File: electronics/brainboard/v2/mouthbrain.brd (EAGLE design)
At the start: 101.6 x 53.3 mm, 28 parts, among them Q1 MOSFET-NCHANNELSMD, Q10 MOSFET-NCHANNELSMD, Q11 MOSFET-NCHANNELSMD, Q12 MOSFET-NCHANNELSMD, Q13 MOSFET-NCHANNELSMD, Q14 MOSFET-NCHANNELSMD, Q15 MOSFET-NCHANNELSMD, Q16 MOSFET-NCHANNELSMD, Q2 MOSFET-NCHANNELSMD, Q3 MOSFET-NCHANNELSMD, Q4 MOSFET-NCHANNELSMD, Q5 MOSFET-NCHANNELSMD, Q6 MOSFET-NCHANNELSMD, Q7 MOSFET-NCHANNELSMD, Q8 MOSFET-NCHANNELSMD, Q9 MOSFET-NCHANNELSMD, U2 ARDUINO-MEGAFULL

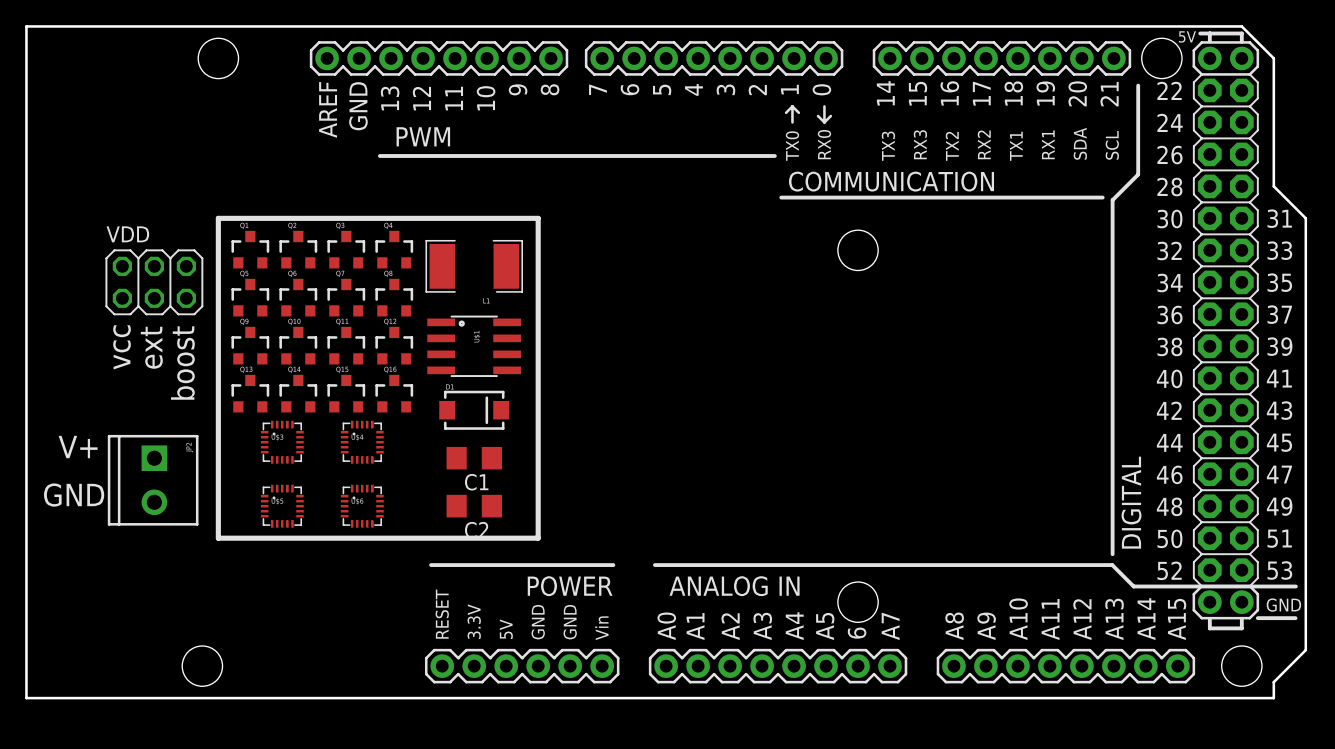
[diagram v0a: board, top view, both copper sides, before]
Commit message: circuit is ready to rock and roll.
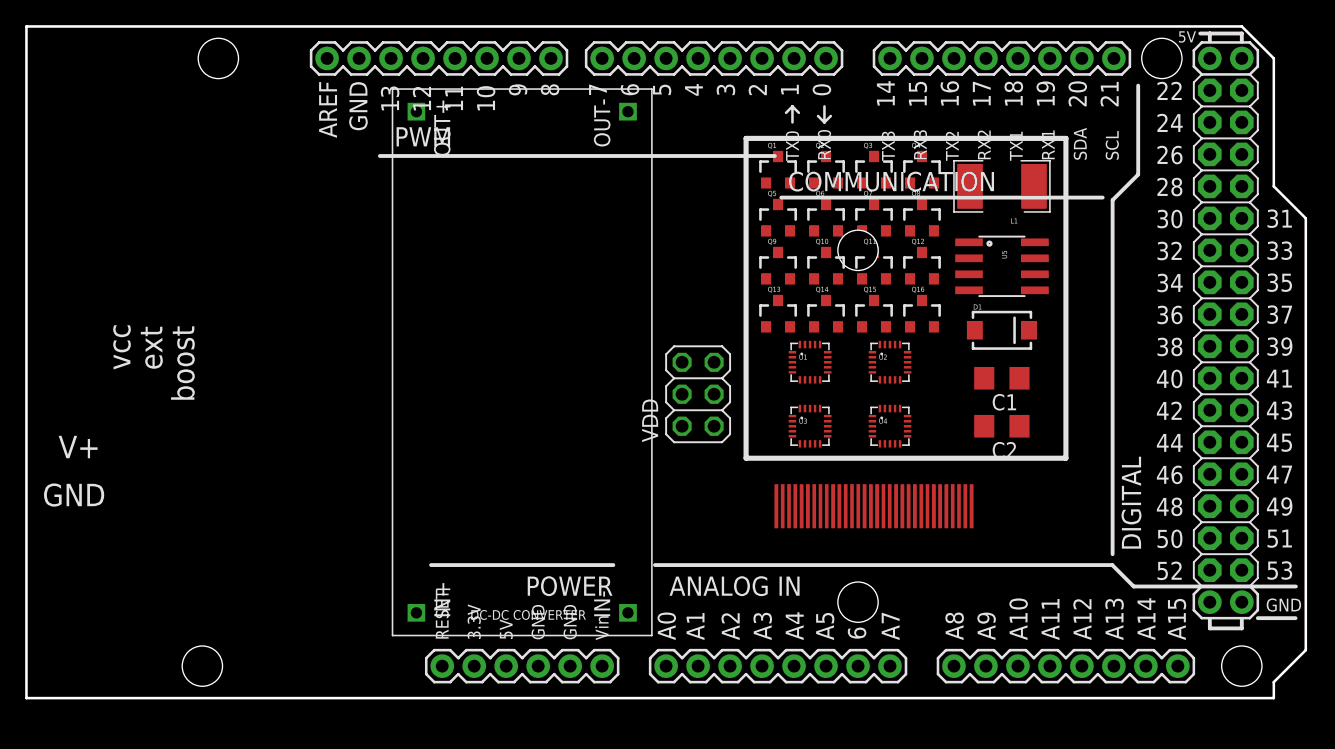
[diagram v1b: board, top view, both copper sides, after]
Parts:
- removed JP2: (no value), SparkFun:SCREWTERMINAL-3.5MM-2
- removed U$3, U$4, U$5, U$6: MCP4352, mouthbrain:QFN-20
- added MEGA: ARDUINO-MEGAFULL, SparkFun:ARDUINO_MEGA
- added U$2: FPC-0.5-32, Hoektronics:FPC-PCB-32
- added U1, U3, U4: MCP4352, mouthbrain:QFN-20
- added U5: MOSFET-NCHANNEL-SOIC8, SparkFun:SO08
- U$1: value MOSFET-NCHANNEL-SOIC8 -> DC-DC-CONVERTER; device SparkFun:SO08 -> Hoektronics:DC-DC-MODULE
- U2: value ARDUINO-MEGAFULL -> MCP4352; device SparkFun:ARDUINO_MEGA -> mouthbrain:QFN-20
- moved U2 73.6 mm to (68.6, 29.2)
- moved VDD 44.1 mm to (53.3, 26.7), turned to 90 degrees
- moved Q11 42.4 mm to (67.3, 36.8)
- moved Q12 42.4 mm to (71.1, 36.8)
- moved Q15 42.4 mm to (67.3, 33.0)
- moved Q16 42.4 mm to (71.1, 33.0)
- moved Q3 42.4 mm to (67.3, 44.5)
- moved Q4 42.4 mm to (71.1, 44.5)
- moved Q7 42.4 mm to (67.3, 40.6)
- moved Q8 42.4 mm to (71.1, 40.6)
- moved C1 42.4 mm to (77.5, 27.9)
- moved C2 42.4 mm to (77.5, 24.1)
- moved D1 42.4 mm to (77.5, 31.8)
- moved L1 42.4 mm to (77.5, 43.2)
- moved Q1 42.4 mm to (59.7, 44.5)
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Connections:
- removed net AN0: Q1.1, U2.22
- removed net AN1: Q2.1, U2.23
- removed net AN10: Q11.1, U2.32
- removed net AN11: Q12.1, U2.33
- removed net AN12: Q13.1, U2.34
- removed net AN13: Q14.1, U2.35
- removed net AN14: Q15.1, U2.36
- removed net AN15: Q16.1
- removed net AN2: Q3.1, U2.24
- removed net AN3: Q4.1, U2.25
- removed net AN4: Q5.1, U2.26
- removed net AN5: Q6.1, U2.27
- removed net AN6: Q7.1, U2.28
- removed net AN7: Q8.1, U2.29
- removed net AN8: Q9.1, U2.30
- removed net AN9: Q10.1, U2.31
- removed net ANODE0: Q1.3
- removed net ANODE1: Q2.3
- removed net ANODE10: Q11.3
- removed net ANODE11: Q12.3
- removed net ANODE12: Q13.3
- removed net ANODE13: Q14.3
- removed net ANODE14: Q15.3
- removed net ANODE15: Q16.3
- removed net ANODE2: Q3.3
- removed net ANODE3: Q4.3
- removed net ANODE4: Q5.3
- removed net ANODE5: Q6.3
- removed net ANODE6: Q7.3
- removed net ANODE7: Q8.3
- removed net ANODE8: Q9.3
- removed net ANODE9: Q10.3
- removed net N$3: C1.1, D1.C
- removed net OUT0: U$3.10, U2.A0
- removed net OUT1: U$3.7, U2.A1
- removed net OUT10: U$5.17, U2.A10
- removed net OUT11: U$5.20, U2.A11
- removed net OUT12: U$6.10, U2.A12
- removed net OUT13: U$6.7, U2.A13
- removed net OUT14: U$6.17, U2.A14
- removed net OUT15: U$6.20, U2.A15
- removed net OUT2: U$3.17, U2.A2
- removed net OUT3: U$3.20, U2.A3
- removed net OUT4: U$4.10, U2.A4
- removed net OUT5: U$4.7, U2.A5
- removed net OUT6: U$4.17, U2.A6
- removed net OUT7: U$4.20, U2.A7
- removed net OUT8: U$5.10, U2.A8
- removed net OUT9: U$5.7, U2.A9
- new net AOUT0: MEGA.A0, U$2.P$2, U1.10
- new net AOUT1: MEGA.A1, U$2.P$4, U1.7
- new net AOUT10: MEGA.A10, U$2.P$22, U3.17
- new net AOUT11: MEGA.A11, U$2.P$24, U3.20
- new net AOUT12: MEGA.A12, U$2.P$26, U4.10
- new net AOUT13: MEGA.A13, U$2.P$28, U4.7
- new net AOUT14: MEGA.A14, U$2.P$30, U4.17
- new net AOUT15: MEGA.A15, U$2.P$32, U4.20
- new net AOUT2: MEGA.A2, U$2.P$6, U1.17
- new net AOUT3: MEGA.A3, U$2.P$8, U1.20
- new net AOUT4: MEGA.A4, U$2.P$10, U2.10
- new net AOUT5: MEGA.A5, U$2.P$12, U2.7
- new net AOUT6: MEGA.A6, U$2.P$14, U2.17
- new net AOUT7: MEGA.A7, U$2.P$16, U2.20
- new net AOUT8: MEGA.A8, U$2.P$18, U3.10
- new net AOUT9: MEGA.A9, U3.7
- new net CIN0: MEGA.22, Q1.1
- new net CIN1: MEGA.23, Q2.1
- new net CIN10: MEGA.32, Q11.1
- new net CIN11: MEGA.33, Q12.1
- new net CIN12: MEGA.34, Q13.1
- new net CIN13: MEGA.35, Q14.1
- new net CIN14: MEGA.36, Q15.1
- new net CIN15: MEGA.37, Q16.1
- new net CIN2: MEGA.24, Q3.1
- new net CIN3: MEGA.25, Q4.1
- new net CIN4: MEGA.26, Q5.1
- new net CIN5: MEGA.27, Q6.1
- new net CIN6: MEGA.28, Q7.1
- new net CIN7: MEGA.29, Q8.1
- new net CIN8: MEGA.30, Q9.1
- new net CIN9: MEGA.31, Q10.1
- new net COUT0: Q1.3, U$2.P$1
- new net COUT1: Q2.3, U$2.P$3
- new net COUT10: Q11.3, U$2.P$21
- new net COUT11: Q12.3, U$2.P$23
- new net COUT12: Q13.3, U$2.P$25
- new net COUT13: Q14.3, U$2.P$27
- new net COUT14: Q15.3, U$2.P$29
- new net COUT15: Q16.3, U$2.P$31
- new net COUT2: Q3.3, U$2.P$5
- new net COUT3: Q4.3, U$2.P$7
- new net COUT4: Q5.3, U$2.P$9
- new net COUT5: Q6.3, U$2.P$11
- new net COUT6: Q7.3, U$2.P$13
- new net COUT7: Q8.3, U$2.P$15
- new net COUT8: Q9.3, U$2.P$17
- new net COUT9: Q10.3, U$2.P$19, U$2.P$20
- net !CS1: now also MEGA.6, U1.2; no longer U$3.2, U2.6
- net !CS2: now also MEGA.7, U2.2; no longer U$4.2, U2.7
- net !CS3: now also MEGA.8, U3.2; no longer U$5.2, U2.8
- net !CS4: now also MEGA.9, U4.2; no longer U$6.2, U2.9
- net !RESET: now also MEGA.2, U1.13, U2.13, U3.13, U4.13; no longer U$3.13, U$4.13, U$5.13, U$6.13, U2.2
- net BOOST: now also C1.1, D1.C
- net BOOST_FET: now also MEGA.11, U5.4; no longer U$1.4
- net EXT: now also U$1.OUT+; no longer JP2.1
- net GND: now also MEGA.GND@0, MEGA.GND@1, MEGA.GND@2, MEGA.GND@3, MEGA.GND@4, U$1.IN-, U$1.OUT-, U1.1, U1.11, U1.16, U1.5, U1.6, U2.1, U2.11, U2.16, U2.5, U2.6, U3.1, U3.11, U3.16, U3.5, U3.6, U4.1, U4.11, U4.16, U4.5, U4.6, U5.5, U5.6, U5.7, U5.8; no longer JP2.2, U$1.5, U$1.6, U$1.7, U$1.8, U$3.5, U$4.5, U$5.5, U$6.5, U2.GND@0, U2.GND@1, U2.GND@2, U2.GND@3, U2.GND@4
- net N$1: now also U5.1, U5.2, U5.3; no longer U$1.1, U$1.2, U$1.3
- net SCK: now also MEGA.3, U1.3, U3.3, U4.3; no longer U$3.3, U$4.3, U$5.3, U$6.3
- net SI: now also MEGA.4, U1.4, U3.4, U4.4; no longer U$3.4, U$4.4, U$5.4, U$6.4
- net SO: now also MEGA.5; no longer U2.5
- net VCC: now also U$1.IN+, U1.15, U2.15, U3.15, U4.15; no longer U$3.15, U$4.15, U$5.15, U$6.15
- net VDD: now also U1.18, U1.19, U1.8, U1.9, U2.18, U2.19, U2.8, U2.9, U3.18, U3.19, U3.8, U3.9, U4.18, U4.19, U4.8, U4.9; no longer U$3.18, U$3.19, U$3.8, U$3.9, U$4.18, U$4.19, U$4.8, U$4.9, U$5.18, U$5.19, U$5.8, U$5.9, U$6.18, U$6.19, U$6.8, U$6.9

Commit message: routed the brainboard
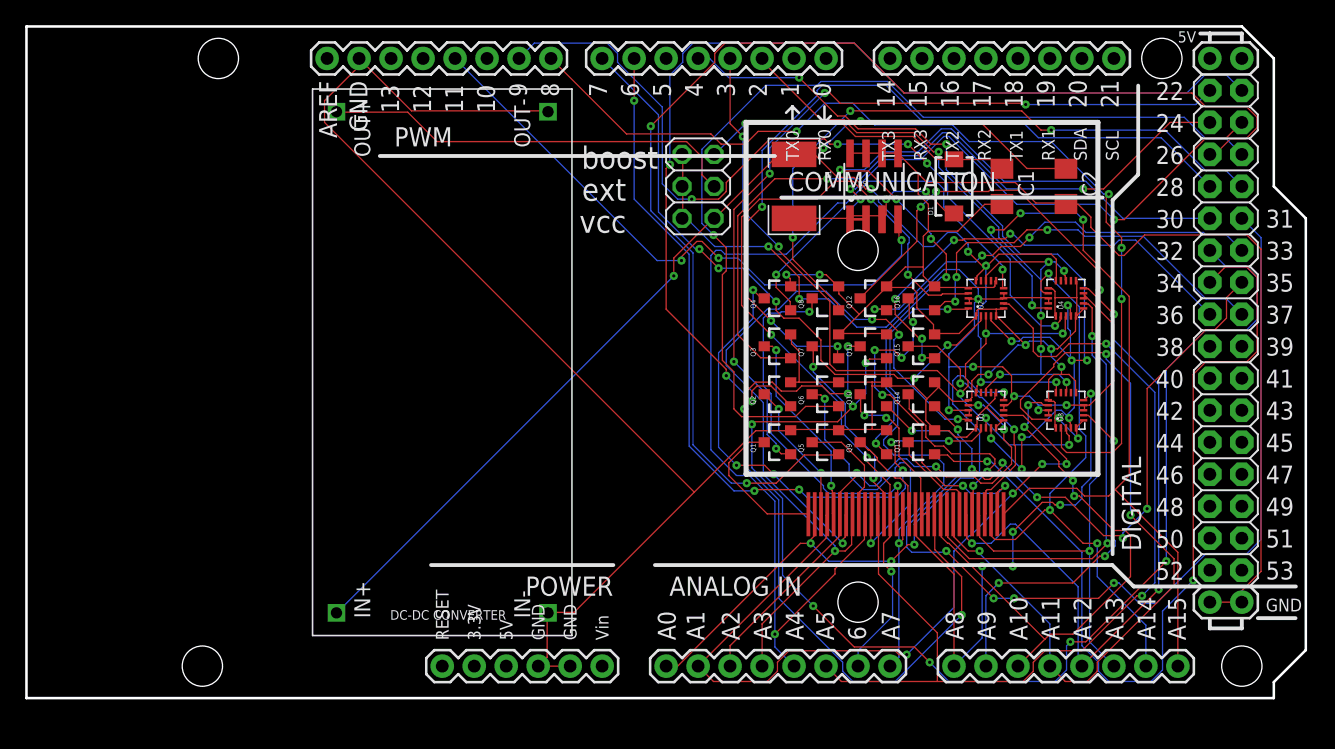
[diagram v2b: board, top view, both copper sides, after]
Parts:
- moved Q1 21.6 mm to (59.7, 22.9), turned to 90 degrees
- moved U3 20.4 mm to (82.5, 25.4), turned to 90 degrees
- moved C2 19.7 mm to (82.5, 43.2), turned to 270 degrees
- moved Q2 18.2 mm to (59.7, 26.7), turned to 90 degrees
- moved Q5 18.2 mm to (63.5, 22.9), turned to 90 degrees
- moved U4 17.3 mm to (82.5, 34.3), turned to 90 degrees
- moved L1 16.5 mm to (61.0, 43.2), turned to 270 degrees
- moved VDD 16.5 mm to (53.3, 43.2)
- moved Q3 15.9 mm to (59.7, 30.5), turned to 90 degrees
- moved Q9 15.9 mm to (67.3, 22.9), turned to 90 degrees
- moved Q13 15.3 mm to (71.1, 22.9), turned to 90 degrees
- moved Q4 15.3 mm to (59.7, 34.3), turned to 90 degrees
- moved C1 15.2 mm to (77.5, 43.2), turned to 270 degrees
- moved U1 14.5 mm to (76.2, 25.4), turned to 90 degrees
- moved Q6 14.0 mm to (63.5, 26.7), turned to 90 degrees
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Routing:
- net GND: track 0.00 -> 308.3 mm, vias 0 -> 8
- net VCC: track 0.00 -> 124.3 mm, vias 0 -> 8
- net CIN4: track 0.00 -> 99.7 mm, vias 0 -> 2
- net CIN10: track 0.00 -> 98.5 mm, vias 0 -> 7
- net VDD: track 0.00 -> 84.4 mm, vias 0 -> 8
- net CIN1: track 0.00 -> 83.2 mm, vias 0 -> 3
- net AOUT4: track 0.00 -> 79.7 mm, vias 0 -> 2
- net !CS3: track 0.00 -> 78.7 mm, vias 0 -> 4
- net SI: track 0.00 -> 78.5 mm, vias 0 -> 10
- net CIN5: track 0.00 -> 78.3 mm, vias 0 -> 1
- net AOUT5: track 0.00 -> 77.5 mm, vias 0 -> 2
- net CIN9: track 0.00 -> 76.5 mm, vias 0 -> 5
- net CIN12: track 0.00 -> 71.6 mm, vias 0 -> 2
- net AOUT6: track 0.00 -> 67.1 mm, vias 0 -> 5
- net SCK: track 0.00 -> 66.6 mm, vias 0 -> 7
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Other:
- board text removed: "GND"
- board text removed: "V+"

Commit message: latest routing
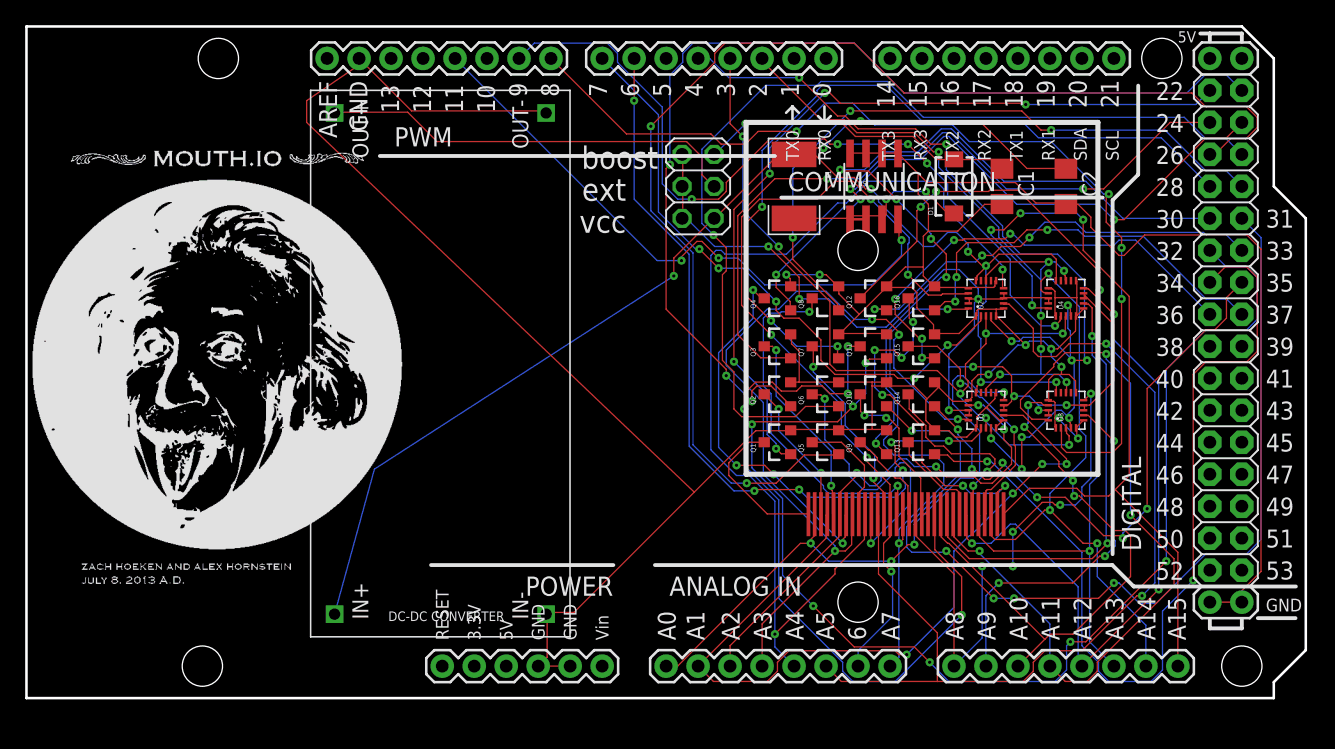
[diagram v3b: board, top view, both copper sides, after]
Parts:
- moved U$1 0.18 mm to (32.9, 29.1)
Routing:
- net GND: track 308.3 -> 310.7 mm
- net VCC: track 124.3 -> 126.7 mm

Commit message: routed a bunch of the brainboard.
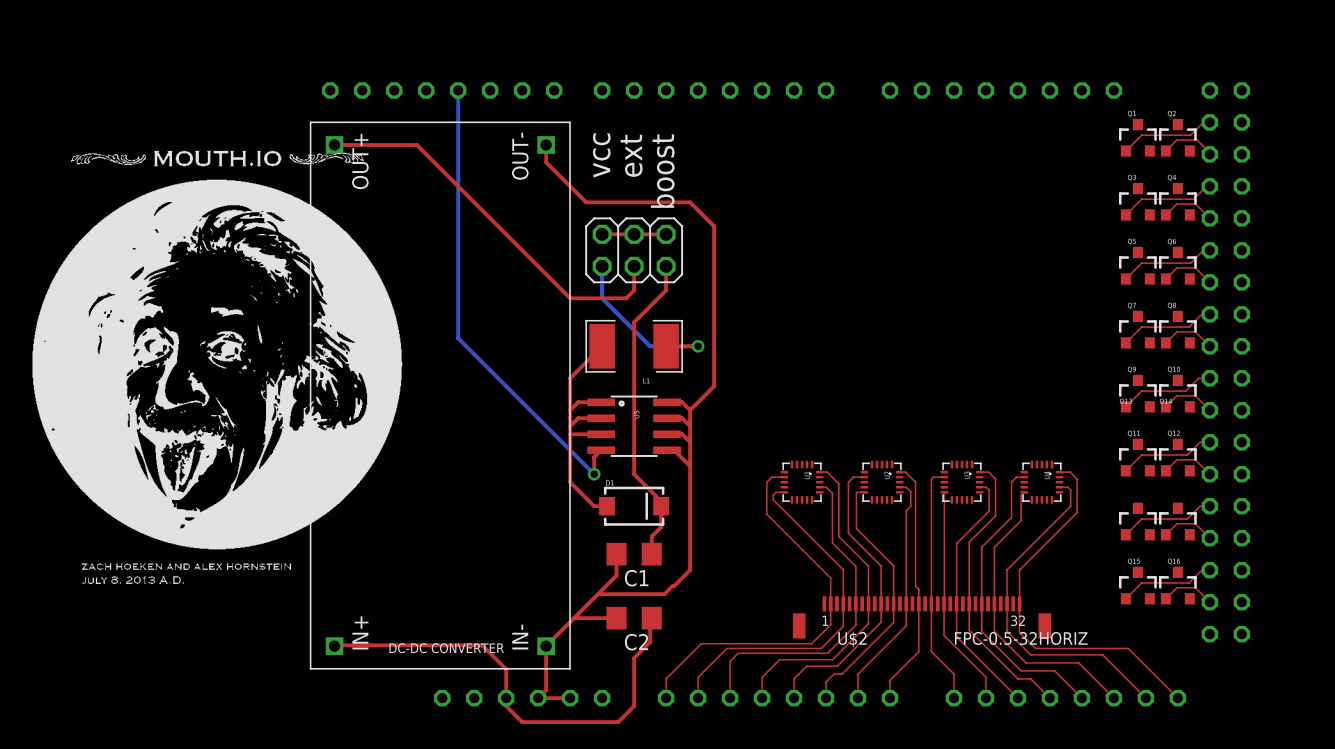
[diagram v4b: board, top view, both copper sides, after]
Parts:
- removed MEGA: ARDUINO-MEGAFULL, SparkFun:ARDUINO_MEGA
- added U$3: ARDUINO-MEGA, Hoektronics:ARDUINO-MEGA
- U$2: value FPC-0.5-32 -> FPC-0.5-32HORIZ; device Hoektronics:FPC-PCB-32 -> Hoektronics:FPC-32-HORIZONTAL
- moved C2 48.5 mm to (48.3, 8.89), turned to 180 degrees
- moved C1 41.3 mm to (48.3, 14.0), turned to 180 degrees
- moved Q2 37.7 mm to (91.4, 47.0), turned to 0 degrees
- moved Q1 37.4 mm to (88.3, 47.0), turned to 0 degrees
- moved D1 35.9 mm to (48.3, 17.8), turned to 0 degrees
- moved Q4 32.7 mm to (91.4, 41.9), turned to 0 degrees
- moved Q3 30.8 mm to (88.3, 41.9), turned to 0 degrees
- moved Q16 30.6 mm to (91.4, 11.4), turned to 0 degrees
- moved Q6 29.7 mm to (91.4, 36.8), turned to 0 degrees
- moved Q5 28.4 mm to (88.3, 36.8), turned to 0 degrees
- moved Q8 28.1 mm to (91.4, 31.8), turned to 0 degrees
- moved Q12 27.3 mm to (91.4, 21.6), turned to 0 degrees
- moved U5 26.9 mm to (48.3, 24.1), turned to 270 degrees
- moved Q15 25.6 mm to (88.3, 11.4), turned to 0 degrees
- moved Q7 24.8 mm to (88.3, 31.8), turned to 0 degrees
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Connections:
- net !CS1: now also U$3.D6; no longer MEGA.6
- net !CS2: now also U$3.D5; no longer MEGA.7
- net !CS3: now also U$3.D4; no longer MEGA.8
- net !CS4: now also U$3.D3; no longer MEGA.9
- net !RESET: now also U$3.D2; no longer MEGA.2
- net AOUT0: now also U$3.A0, U1.7; no longer MEGA.A0, U1.10
- net AOUT1: now also U$3.A1, U1.10; no longer MEGA.A1, U1.7
- net AOUT10: now also U$3.A10; no longer MEGA.A10
- net AOUT11: now also U$3.A11; no longer MEGA.A11
- net AOUT12: now also U$3.A12, U4.7; no longer MEGA.A12, U4.10
- net AOUT13: now also U$3.A13, U4.10; no longer MEGA.A13, U4.7
- net AOUT14: now also U$3.A14; no longer MEGA.A14
- net AOUT15: now also U$3.A15; no longer MEGA.A15
- net AOUT2: now also U$3.A2; no longer MEGA.A2
- net AOUT3: now also U$3.A3; no longer MEGA.A3
- net AOUT4: now also U$3.A4, U2.7; no longer MEGA.A4, U2.10
- net AOUT5: now also U$3.A5, U2.10; no longer MEGA.A5, U2.7
- net AOUT6: now also U$3.A6; no longer MEGA.A6
- net AOUT7: now also U$3.A7; no longer MEGA.A7
- net AOUT8: now also U$3.A8, U3.7; no longer MEGA.A8, U3.10
- net AOUT9: now also U$2.P$20, U$3.A9, U3.10; no longer MEGA.A9, U3.7
- net BOOST_FET: now also U$3.D11; no longer MEGA.11
- net CIN0: now also U$3.D22; no longer MEGA.22
- net CIN1: now also U$3.D24; no longer MEGA.23
- net CIN10: now also U$3.D42; no longer MEGA.32
- net CIN11: now also U$3.D44; no longer MEGA.33
- net CIN12: now also U$3.D46; no longer MEGA.34
- net CIN13: now also U$3.D48; no longer MEGA.35
- net CIN14: now also U$3.D50; no longer MEGA.36
- net CIN15: now also U$3.D52; no longer MEGA.37
- net CIN2: now also U$3.D26; no longer MEGA.24
- net CIN3: now also U$3.D28; no longer MEGA.25
- net CIN4: now also U$3.D30; no longer MEGA.26
- net CIN5: now also U$3.D32; no longer MEGA.27
- net CIN6: now also U$3.D34; no longer MEGA.28
- net CIN7: now also U$3.D36; no longer MEGA.29
- net CIN8: now also U$3.D38; no longer MEGA.30
- net CIN9: now also U$3.D40; no longer MEGA.31
- net COUT9: no longer U$2.P$20
- net GND: now also U$3.GND4, U$3.GND5; no longer MEGA.GND@0, MEGA.GND@1, MEGA.GND@2, MEGA.GND@3, MEGA.GND@4
- net SCK: now also U$3.D7; no longer MEGA.3
- net SI: now also U$3.D8; no longer MEGA.4
- net SO: now also U$3.D9; no longer MEGA.5
- net VCC: now also U$3.5V-3
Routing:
- net GND: track 310.7 -> 81.6 mm, vias 8 -> 0
- net CIN4: track 99.7 -> 7.61 mm, vias 2 -> 0
- net CIN10: track 98.5 -> 7.61 mm, vias 7 -> 0
- net VDD: track 84.4 -> 5.08 mm, vias 8 -> 0
- net CIN1: track 83.2 -> 4.40 mm, vias 3 -> 0
- net !CS3: track 78.7 -> 0.00 mm, vias 4 -> 0
- net SI: track 78.5 -> 0.00 mm, vias 10 -> 0
- net VCC: track 126.7 -> 50.4 mm, vias 8 -> 1
- net CIN5: track 78.3 -> 4.33 mm, vias 1 -> 0
- net CIN9: track 76.5 -> 4.33 mm, vias 5 -> 0
- net SCK: track 66.6 -> 0.00 mm, vias 7 -> 0
- net COUT11: track 64.3 -> 0.00 mm, vias 4 -> 0
- net !CS4: track 64.0 -> 0.00 mm, vias 5 -> 0
- net CIN12: track 71.6 -> 7.61 mm, vias 2 -> 0
- net !CS1: track 63.7 -> 0.00 mm, vias 6 -> 0
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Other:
- board outline removed
